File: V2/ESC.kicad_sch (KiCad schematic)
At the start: 86 parts, among them IC1 DRV8302DCA, IC2 TPS54331DR, J1 Conn_01x01, J2 Conn_01x01, J3 Conn_01x01, J5 Conn_ALIM_MOTOR, J6 USB_C_Receptacle_USB2.0, Q1 2N7002, U1 ATmega328P-AU_full, U2 FT230XS, Y1 CSTCE

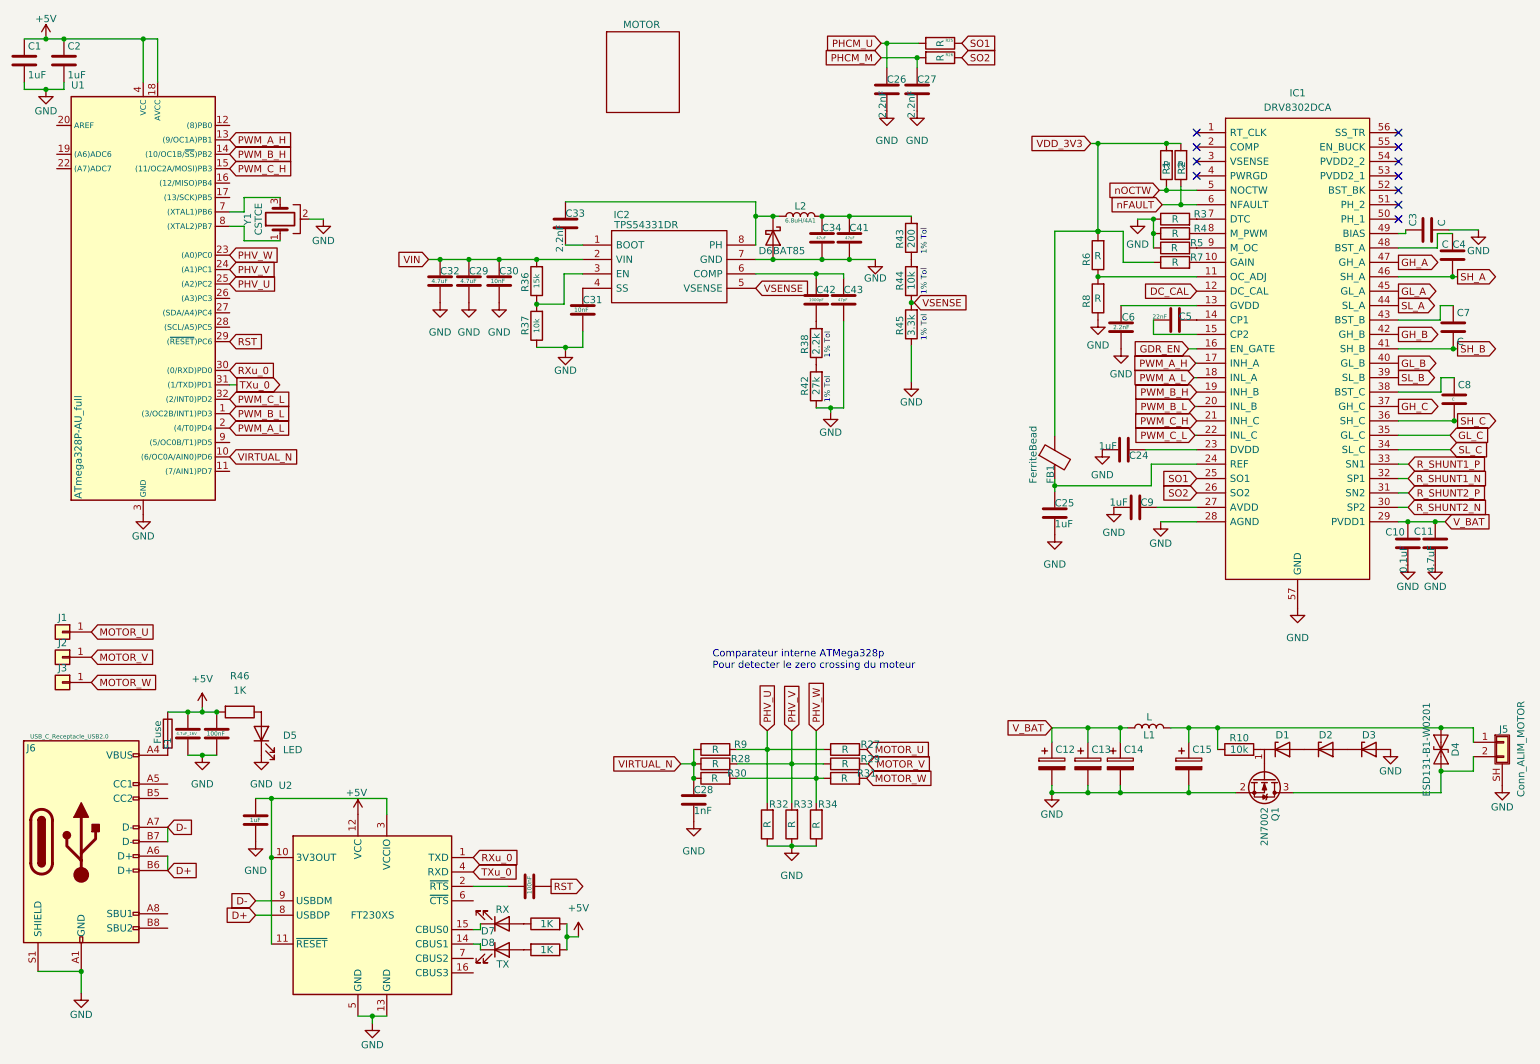
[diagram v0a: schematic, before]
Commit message: def
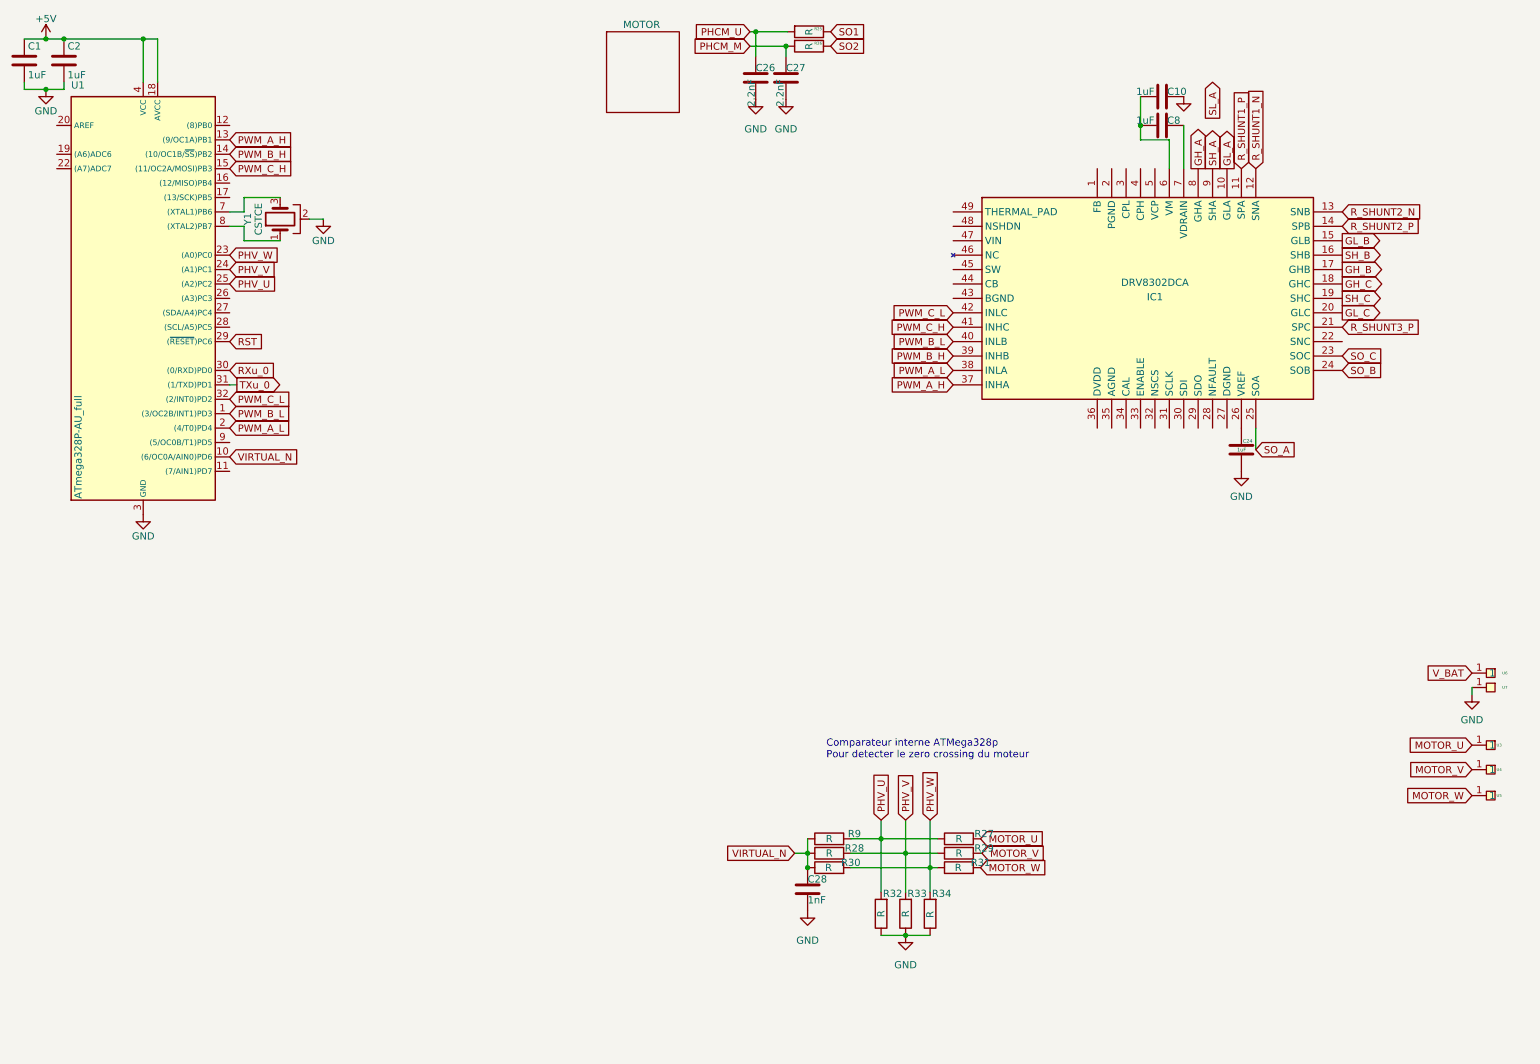
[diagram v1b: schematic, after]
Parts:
- removed 6.8uH/4A1: L2, Inductor_SMD:L_1206_3216Metric, symbol Device:L
- removed C11, C29, C32: 4.7uF, Capacitor_SMD:C_1206_3216Metric, symbol Device:C
- removed C12, C13, C14, C15: C_Polarized, Capacitor_SMD:CP_Elec_4x3, symbol Device:C_Polarized
- removed C25, C9: 1uF, Capacitor_SMD:C_1206_3216Metric, symbol Device:C
- removed C3, C4, C7: C, Capacitor_SMD:C_1206_3216Metric, symbol Device:C
- removed C30, C31: 10nF, Capacitor_SMD:C_1206_3216Metric, symbol Device:C
- removed C33, C6: 2.2nF, Capacitor_SMD:C_1206_3216Metric, symbol Device:C
- removed C34, C41: 47uF, Capacitor_SMD:C_1206_3216Metric, symbol Device:C
- removed C42: 1000pF, Capacitor_SMD:C_1206_3216Metric, symbol Device:C
- removed C43: 47pF, Capacitor_SMD:C_1206_3216Metric, symbol Device:C
- removed C44: 1uF, Capacitor_SMD:C_1206_3216Metric_Pad1.33x1.80mm_HandSolder, symbol Device:C
- removed C45: 4.7uF_16V, Capacitor_SMD:C_1206_3216Metric_Pad1.33x1.80mm_HandSolder, symbol Device:C
- removed C46, C47: 100nF, Capacitor_SMD:C_1206_3216Metric_Pad1.33x1.80mm_HandSolder, symbol Device:C
- removed C5: 22nF, Capacitor_SMD:C_1206_3216Metric, symbol Device:C
- removed D1, D2, D3: ZMMxx, Diode_SMD:D_MiniMELF, symbol Diode:ZMMxx
- removed D4: ESD131-B1-W0201, Diode_SMD:Infineon_SG-WLL-2-3_0.58x0.28_P0.36mm, symbol Diode:ESD131-B1-W0201
- removed D5: LED, LED_SMD:LED_1206_3216Metric_Pad1.42x1.75mm_HandSolder, symbol Device:LED
- removed D6: BAT85, Diode_THT:D_DO-35_SOD27_P7.62mm_Horizontal, symbol Diode:BAT85
- removed D7: RX, LED_SMD:LED_1206_3216Metric_Pad1.42x1.75mm_HandSolder, symbol Device:LED
- removed D8: TX, LED_SMD:LED_1206_3216Metric_Pad1.42x1.75mm_HandSolder, symbol Device:LED
- removed F1: Fuse, Fuse:Fuse_1206_3216Metric_Pad1.42x1.75mm_HandSolder, symbol Device:Fuse
- removed FB1: FerriteBead, Inductor_SMD:L_1206_3216Metric, symbol Device:FerriteBead
- removed IC1: DRV8302DCA, Dam_libkicad:SOP50P810X120-57N, symbol Dam_libkicad:DRV8302DCA
- removed IC2: TPS54331DR, Dam_libkicad:SOIC127P600X175-8N, symbol Dam_libkicad:TPS54331DR
- removed J1, J2, J3: Conn_01x01, Connector_JST:JST_ACH_BM01B-ACHSS-A-GAN-ETF_1x01-1MP_P1.20mm_Vertical, symbol Connector_Generic:Conn_01x01
- removed J5: Conn_ALIM_MOTOR, symbol Connector_Generic_Shielded:Conn_01x02_Shielded
- removed J6: USB_C_Receptacle_USB2.0, Connector_USB:USB_C_Receptacle_GCT_USB4105-xx-A_16P_TopMnt_Horizontal, symbol Connector:USB_C_Receptacle_USB2.0
- removed L1: L, Inductor_SMD:L_1206_3216Metric, symbol Device:L
- removed Q1: 2N7002, Package_TO_SOT_SMD:SOT-23, symbol Transistor_FET:2N7002
- removed R1, R2, R3, R4, R5, R6, R7, R8: R, Resistor_SMD:R_1206_3216Metric, symbol Device:R
- removed R10, R37, R44: 10k, Resistor_SMD:R_1206_3216Metric, symbol Device:R
- removed R36: 15k, Resistor_SMD:R_1206_3216Metric, symbol Device:R
- removed R38: 2.2k, Resistor_SMD:R_1206_3216Metric, symbol Device:R
- removed R42: 27k, Resistor_SMD:R_1206_3216Metric, symbol Device:R
- removed R43: 200, Resistor_SMD:R_1206_3216Metric, symbol Device:R
- removed R45: 3.3k, Resistor_SMD:R_1206_3216Metric, symbol Device:R
- removed R46, R47, R48: 1K, Resistor_SMD:R_1206_3216Metric_Pad1.30x1.75mm_HandSolder, symbol Device:R
- removed U2: FT230XS, Package_SO:SSOP-16_5.3x6.2mm_P0.65mm, symbol Interface_USB:FT230XS
- added IC1: DRV8302DCA, Dam_libkicad:QFN50P700X700X100-49N-D, symbol Dam_libkicad:DRV8323RSRGZT
- added U3, U4, U5, U6, U7: ~, Dam_libkicad:PAD_Connector, symbol Dam_libkicad:PAD_Connector
- C1, C2: footprint Dam_libkicad:1206 -> Dam_libkicad:0603
- C10: value 0.1uF -> 1uF; footprint Capacitor_SMD:C_1206_3216Metric -> Dam_libkicad:0603
- C24, C26, C27, C28: footprint Capacitor_SMD:C_1206_3216Metric -> Dam_libkicad:0603
- C8: value C -> 1uF; footprint Capacitor_SMD:C_1206_3216Metric -> Dam_libkicad:0603
- R25, R26, R27, R28, R29, R30, R31, R32, R33, R34, R9: footprint Resistor_SMD:R_1206_3216Metric -> Dam_libkicad:0603
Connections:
- net GH_A: now also IC1.8 (GHA)
- net GH_B: now also IC1.17 (GHB)
- net GH_C: now also IC1.18 (GHC)
- net GL_A: now also IC1.10 (GLA)
- net GL_B: now also IC1.15 (GLB)
- net GL_C: now also IC1.20 (GLC)
- net GND: now also C10.1, U7.1; no longer C10.2
- net MOTOR_U: now also U3.1
- net MOTOR_V: now also U4.1
- net MOTOR_W: now also U5.1
- net PWM_A_H: now also IC1.37 (INHA)
- net PWM_A_L: now also IC1.38 (INLA)
- net PWM_B_H: now also IC1.39 (INHB)
- net PWM_B_L: now also IC1.40 (INLB)
- net PWM_C_H: now also IC1.41 (INHC)
- net PWM_C_L: now also IC1.42 (INLC)
- net R_SHUNT1_N: now also IC1.12 (SNA)
- net R_SHUNT1_P: now also IC1.11 (SPA)
- net R_SHUNT2_N: now also IC1.13 (SNB)
- net R_SHUNT2_P: now also IC1.14 (SPB)
- net SH_A: now also IC1.9 (SHA)
- net SH_B: now also IC1.16 (SHB)
- net SH_C: now also IC1.19 (SHC); no longer C8.2
- net V_BAT: now also U6.1; no longer C10.1
- net at C24.1: now also IC1.26 (VREF)
- net at C8.1: now also IC1.7 (VDRAIN)
- new net: C10.2, C8.2, IC1.6 (VM)
- new net R_SHUNT3_P: IC1.21 (SPC)
- new net SO_A: IC1.25 (SOA)
- new net SO_B: IC1.24 (SOB)
- new net SO_C: IC1.23 (SOC)
- no-connect marks 11 -> 0
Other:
- note removed: "1% Tol"
- moved on the sheet: C24, C26, C27, C28, R25, R26, R27, R28, R29, R30, R31, R32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
